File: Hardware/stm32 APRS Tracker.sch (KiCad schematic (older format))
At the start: 75 parts, among them IC1 STM32F103x, P1 USB_B, P101 CONN_01X04, P102 CONN_01X04, P103 CONN_01X01, SW101 SW_TxPwr, U1 AP1117D33, U101 STM32_mmvisual_JTAG, U2 SP0503BAHTG, Y101 8 MHz, Y102 32,768

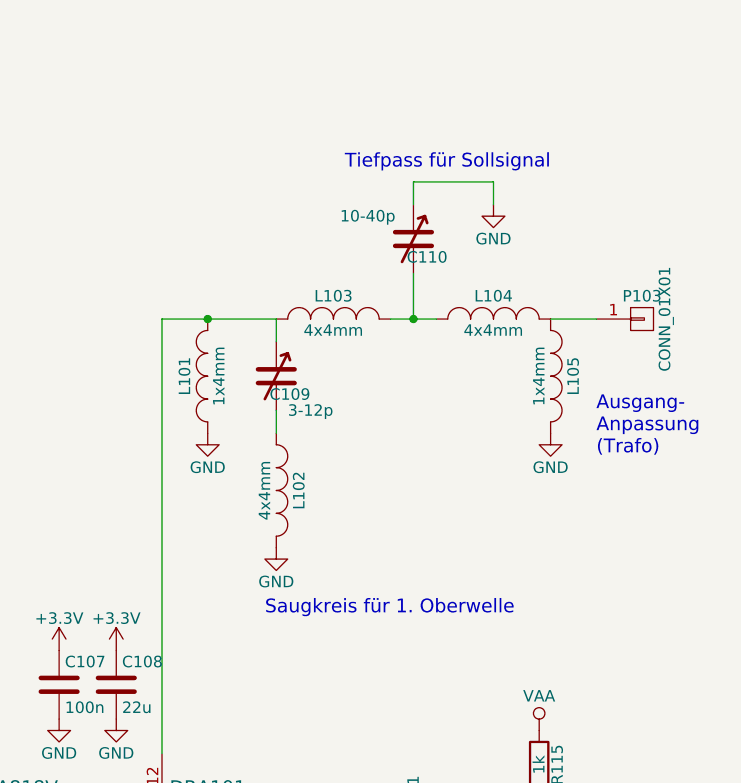
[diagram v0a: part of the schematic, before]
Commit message: Platine bis auf Sicherung fertig
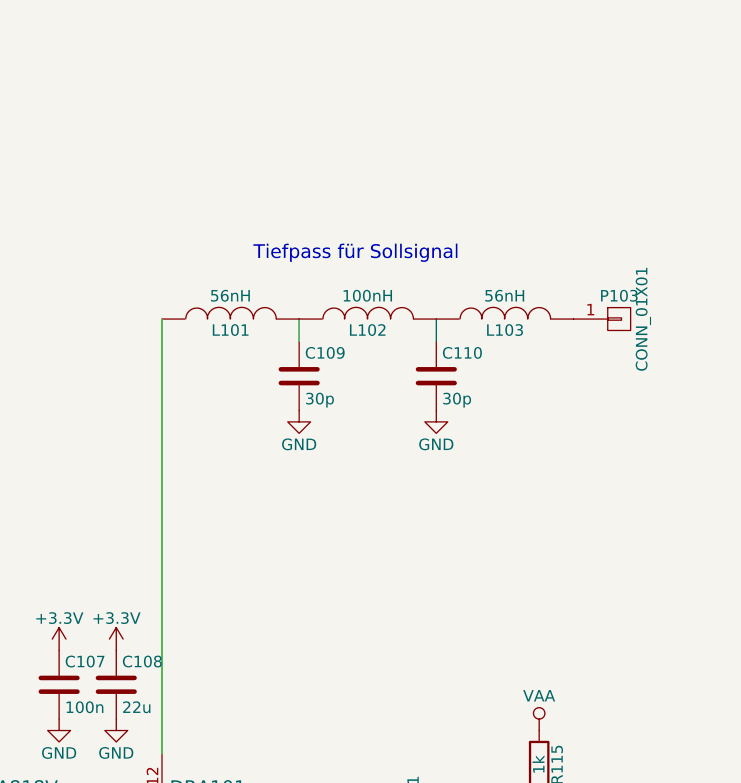
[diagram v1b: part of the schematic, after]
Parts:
- removed C109: 3-12p, symbol CTRIM
- removed C110: 10-40p, symbol CTRIM
- removed L101, L105: 1x4mm, symbol INDUCTOR_SMALL
- removed L102, L103, L104: 4x4mm, symbol INDUCTOR_SMALL
- added C109, C110: 30p, Capacitors_SMD:C_0402, symbol C
- added L101, L103: 56nH, Resistors_SMD:R_0402, symbol INDUCTOR
- added L102: 100nH, Resistors_SMD:R_0402, symbol INDUCTOR
- BT101: footprint (none) -> Pin_Headers:Pin_Header_Angled_1x02
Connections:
- net GND: now also C109.2, C110.2
- net at DRA101.12 (Antenna): now also L101.1
- net at P103.1 (P1): now also L103.2
- new net: C109.1, L101.2, L102.1
- new net: C110.1, L102.2, L103.1
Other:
- note removed: "Ausgang-\nAnpassung\n(Trafo)"
- note removed: "Saugkreis für 1. Oberwelle"
- moved on the sheet: P103
